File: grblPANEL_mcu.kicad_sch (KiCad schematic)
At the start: 31 parts, among them J201 2x5x1.27mm, J202 USB_C_Receptacle_USB2.0, SW201 SW_Push, SW202 SW_Push, U201 STM32G0B1CxTxN, U202 USBLC6-2SC6, Y201 8MHz

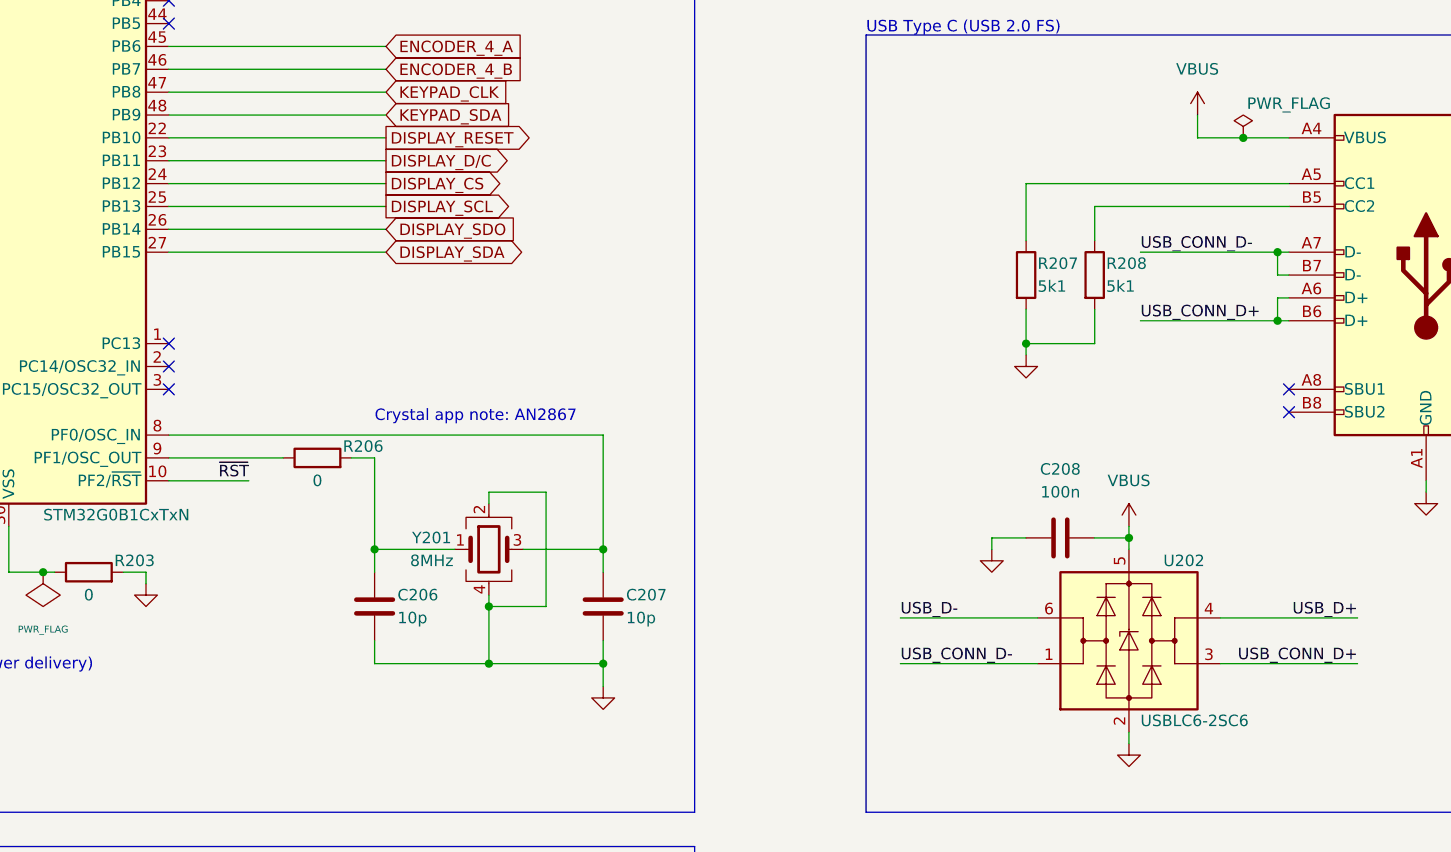
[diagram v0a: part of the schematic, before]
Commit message: Weeny schematic update
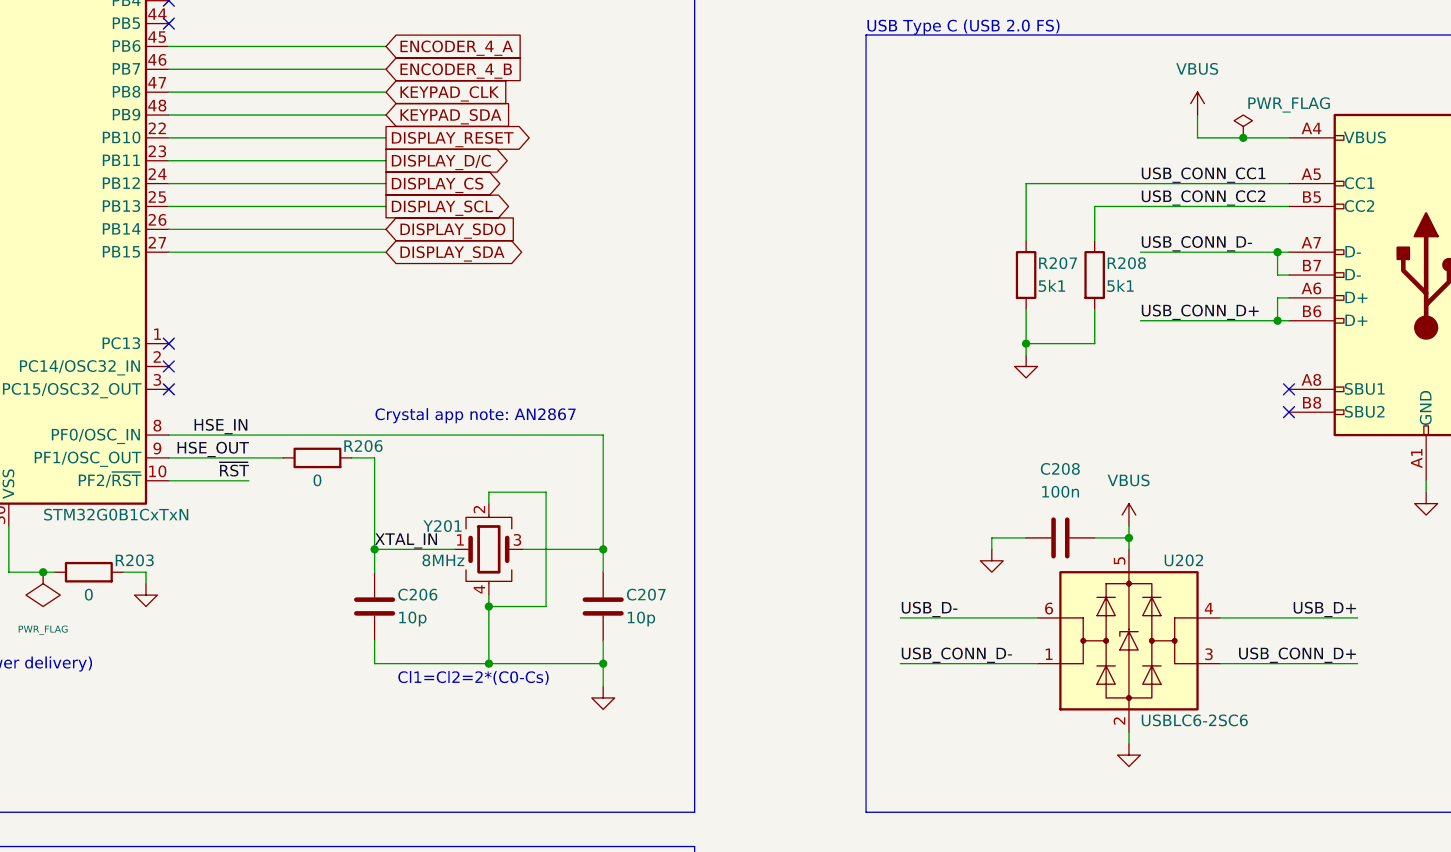
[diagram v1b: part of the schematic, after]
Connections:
- net USB_CONN_CC1: now reaches J202.A5 (CC1), R207.1
- net USB_CONN_CC2: now reaches J202.B5 (CC2), R208.1
- net HSE_IN: now reaches C207.1, U201.8 (PF0/OSC_IN), Y201.3
- net XTAL_IN: now reaches C206.1, R206.2, Y201.1
- net HSE_OUT: now reaches R206.1, U201.9 (PF1/OSC_OUT)
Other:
- note added: "Cl1=Cl2=2*(C0-Cs)"
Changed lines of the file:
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@@
+    (effects (font (size 1.27 1.27)) (justify left bottom))
+  )
+  (text "Cl1=Cl2=2*(C0-Cs)" (at 142.24 147.32 0)
     (effects (font (size 1.27 1.27)) (justify left bottom))
   )
@@
     (effects (font (size 1.27 1.27)) (justify right bottom))
   )
+  (label "XTAL_IN" (at 139.7 132.08 0)
+    (effects (font (size 1.27 1.27)) (justify left bottom))
+  )
   (label "USB_D-" (at 63.5 96.52 0)
     (effects (font (size 1.27 1.27)) (justify left bottom))
   )
+  (label "HSE_IN" (at 125.73 119.38 180)
+    (effects (font (size 1.27 1.27)) (justify right bottom))
+  )
   (label "USB_CONN_D-" (at 224.79 99.06 0)
     (effects (font (size 1.27 1.27)) (justify left bottom))
   )
+  (label "USB_CONN_CC2" (at 224.79 93.98 0)
+    (effects (font (size 1.27 1.27)) (justify left bottom))
+  )
   (label "USB_CONN_D+" (at 248.92 144.78 180)
     (effects (font (size 1.27 1.27)) (justify right bottom))
@@
     (effects (font (size 1.27 1.27)) (justify left bottom))
   )
+  (label "USB_CONN_CC1" (at 224.79 91.44 0)
+    (effects (font (size 1.27 1.27)) (justify left bottom))
+  )
   (label "USB_CONN_D-" (at 198.12 144.78 0)
     (effects (font (size 1.27 1.27)) (justify left bottom))
@@
   (label "SWCLK{slash}BOOT0" (at 44.45 181.61 0)
     (effects (font (size 1.27 1.27)) (justify left bottom))
+  )
+  (label "HSE_OUT" (at 125.73 121.92 180)
+    (effects (font (size 1.27 1.27)) (justify right bottom))
   )
   (label "~{RST}" (at 273.05 46.99 180)
@@
   (symbol (lib_id "Device:Crystal_GND24") (at 152.4 132.08 0) (unit 1)
     (in_bom yes) (on_board yes)
-    (property "Reference" "Y201" (id 0) (at 146.05 130.81 0))
-    (property "Value" "8MHz" (id 1) (at 146.05 133.35 0))
+    (property "Reference" "Y201" (id 0) (at 147.32 129.54 0))
+    (property "Value" "8MHz" (id 1) (at 147.32 133.35 0))
     (property "Footprint" "Crystal:Crystal_SMD_3225-4Pin_3.2x2.5mm" (id 2) (at 152.4 132.08 0)
       (effects (font (size 1.27 1.27)) hide)
